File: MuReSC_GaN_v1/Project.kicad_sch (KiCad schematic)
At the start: 115 parts, among them IC1 STM32G474RET6, IC10 UCC12040DVE, IC11 LMG1020YFFR, IC12 LMG1020YFFR, IC13 LMG1020YFFR, IC14 LMG1020YFFR, IC2 TPSM5601R5HRDAR, IC3 ISO7720FQDQ1, IC4 ISO7720FQDQ1, IC5 ISO7720FQDQ1, IC6 ISO7720FQDQ1, IC7 UCC12040DVE, IC8 UCC12040DVE, IC9 UCC12040DVE, J1 62000211121_x6, J2 62000211121, J3 62000211121_x1, J4 62000211121_x1, P1 691214110002, P2 691214110002, Q1 GS61004B-TR, Q2 GS61004B-TR, Q3 GS61004B-TR, Q4 GS61004B-TR, Y1 NX3215SA-32.768K-STD-MUS-2, Y2 NX3225SA-24.000MHZ-STD-CSR-1

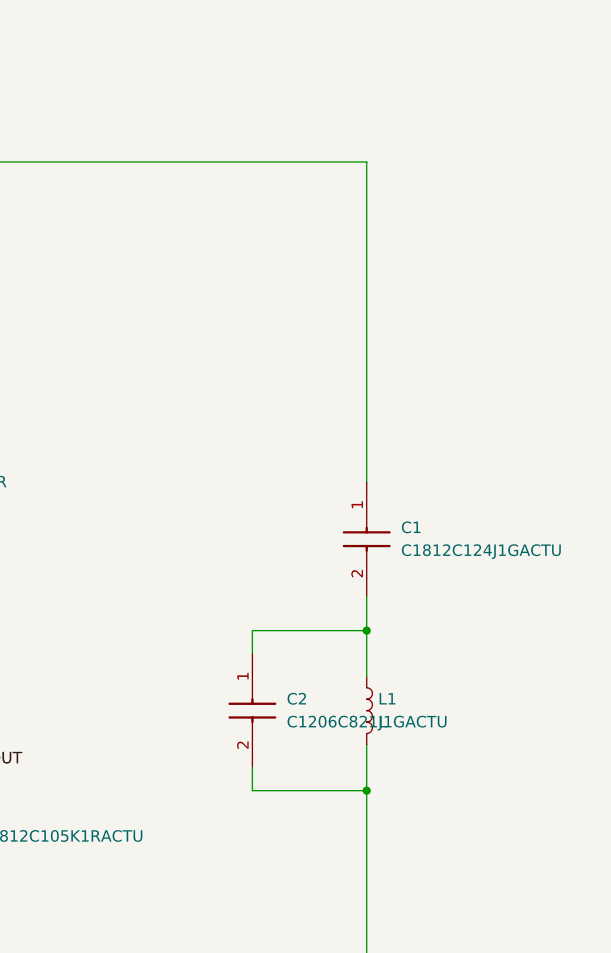
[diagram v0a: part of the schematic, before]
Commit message: placement
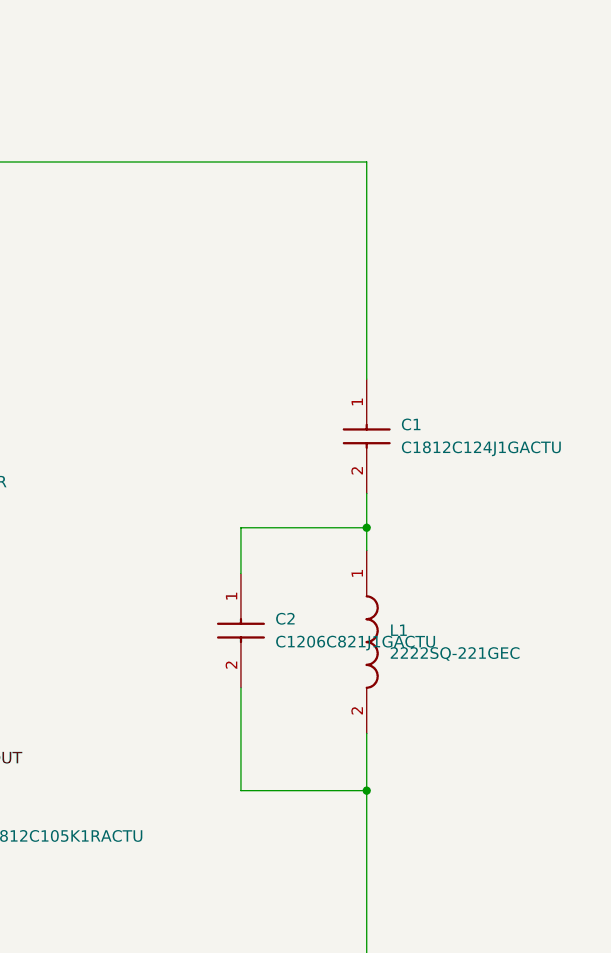
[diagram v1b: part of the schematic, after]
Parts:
- removed L1: L, Inductor_SMD:L_0603_1608Metric, symbol Device:L
- added L1: 2222SQ-221GEC, 2222SQ221GEC, symbol SamacSys_Parts:2222SQ-221GEC
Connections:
- net S3: now also L1.2
- net at C1.2, C2.1: now also L1.1
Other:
- moved on the sheet: C1, C2
